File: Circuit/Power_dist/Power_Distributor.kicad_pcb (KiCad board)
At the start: 2 copper layers, 150.2 x 108.9 mm, 97 parts, among them CON1 Conn-PCIE-x16, J1 Thruster_Off_Switch, P1 XT60, P11 XT60, P15 USB_B, P16 XT60, P17 XT60, P2 XT30, P3 XT30, P4 XT30, P5 XT30, Q1 IPD90P03P4L, Q2 IPD90P03P4L, Q3 IPD90P03P4L, Q5 IPD90P03P4L, Q6 AUIRFS8409-7P, Q7 AUIRFS8409-7P, U1 93LC56BT-I/OT, U2 FT232H, U3 ACPL-247-500E, U4 ACPL-247-500E, U5 LTC4357, U6 LTC4357, U7 UWE-12/6-Q12P, U8 TEN_20-2411WIN, Y1 12MHz

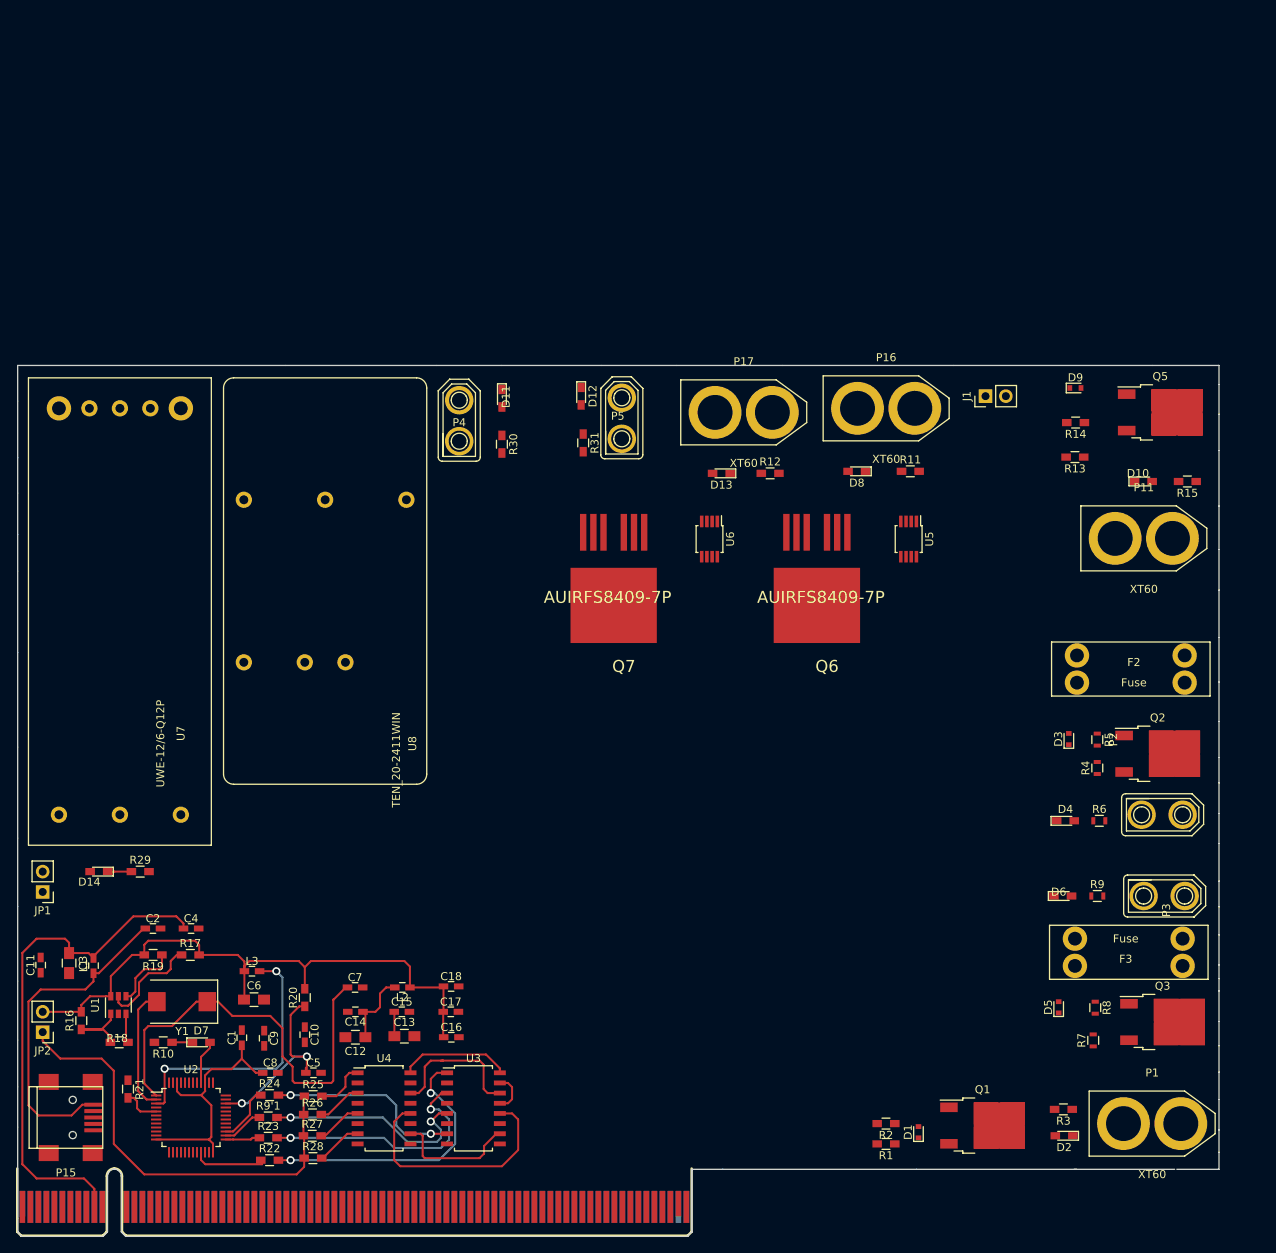
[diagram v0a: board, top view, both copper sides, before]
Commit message: route pcb except gnd
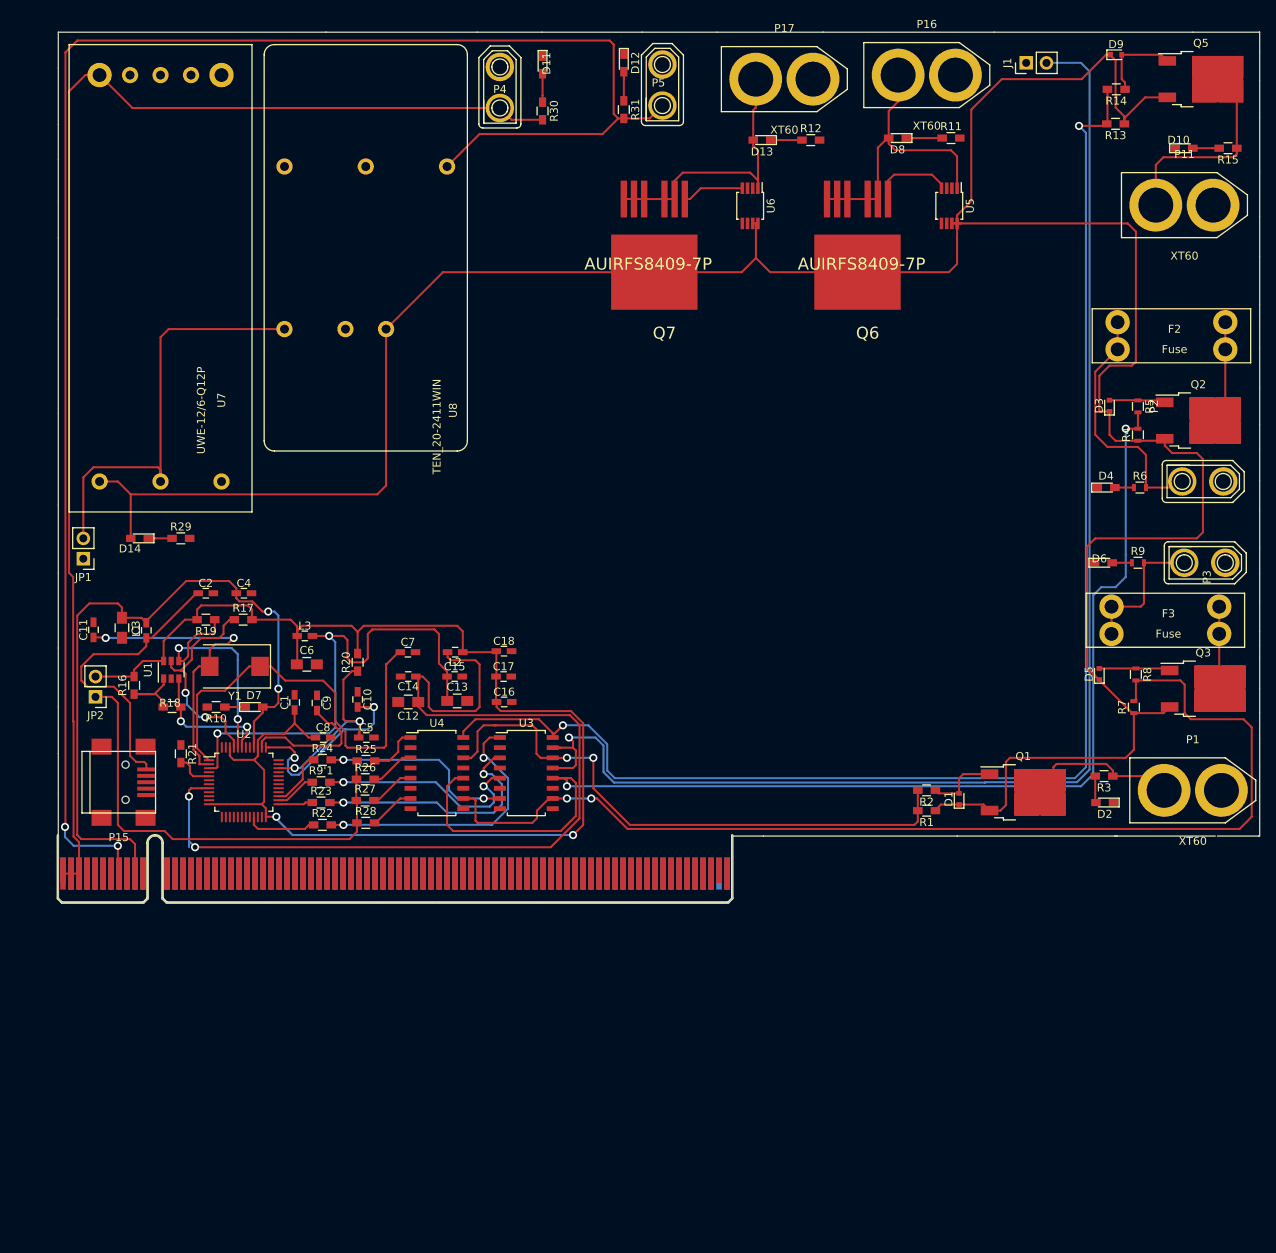
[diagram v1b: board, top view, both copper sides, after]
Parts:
- moved C13 42.4 mm to (100.3, 116.6)
- moved C14 42.4 mm to (94.2, 113.5)
- moved C15 42.4 mm to (100.0, 113.5)
- moved C17 42.4 mm to (106.1, 113.5)
- moved C3 42.4 mm to (58.4, 107.4)
- moved C5 42.4 mm to (89.0, 121.2)
- moved C6 42.4 mm to (81.5, 112.0)
- moved C7 42.4 mm to (94.2, 110.5)
- moved C8 42.4 mm to (83.6, 121.2)
- moved D7 42.4 mm to (74.9, 117.3)
- moved L2 42.4 mm to (100.1, 110.5)
- moved P15 42.4 mm to (58.7, 126.7)
- moved R10 42.4 mm to (70.2, 117.3)
- moved R17 42.4 mm to (73.6, 106.4)
- moved R18 42.4 mm to (64.7, 117.3)
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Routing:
- net +BATT: track 0.00 -> 356.9 mm
- net +5V: track 0.00 -> 218.3 mm, vias 0 -> 2
- net /Kill_SW: track 5.00 -> 174.6 mm, vias 0 -> 1
- net +12V: track 0.00 -> 165.6 mm
- net /Power_Controller/SW1_C: track 14.3 -> 175.4 mm, vias 0 -> 2
- net /Power_Controller/SW4_C: track 15.8 -> 138.2 mm, vias 0 -> 2
- net /Power_Controller/SW3_C: track 30.8 -> 152.7 mm, vias 0 -> 2
- net Net-(C12-Pad1): track 9.53 -> 119.1 mm, vias 0 -> 2
- net +3V3: track 108.7 -> 175.0 mm, vias 0 -> 2
- net /Power_Controller/SW2_C: track 18.1 -> 73.5 mm, vias 0 -> 2
- net Net-(JP1-Pad2): track 0.00 -> 53.3 mm
- net Net-(D8-Pad2): track 0.00 -> 36.9 mm
- net Net-(D13-Pad2): track 0.00 -> 33.9 mm
- net Net-(F2-Pad2): track 0.00 -> 31.5 mm
- net Net-(C13-Pad1): track 37.3 -> 63.2 mm
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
